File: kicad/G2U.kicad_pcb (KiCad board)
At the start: 2 copper layers, 78 x 71.4 mm, 38 parts, among them J1 Conn_02x12_Counter_Clockwise_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

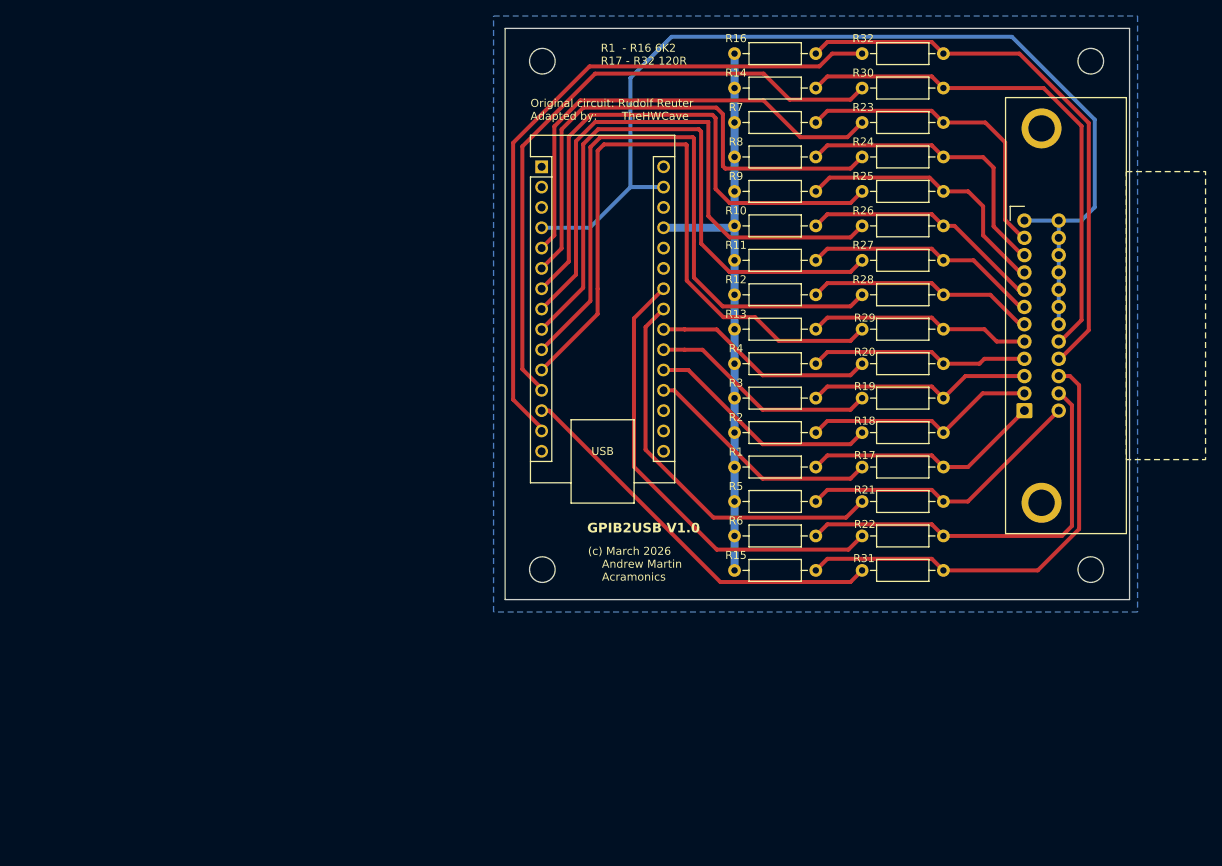
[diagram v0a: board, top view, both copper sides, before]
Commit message: Final 0603 board
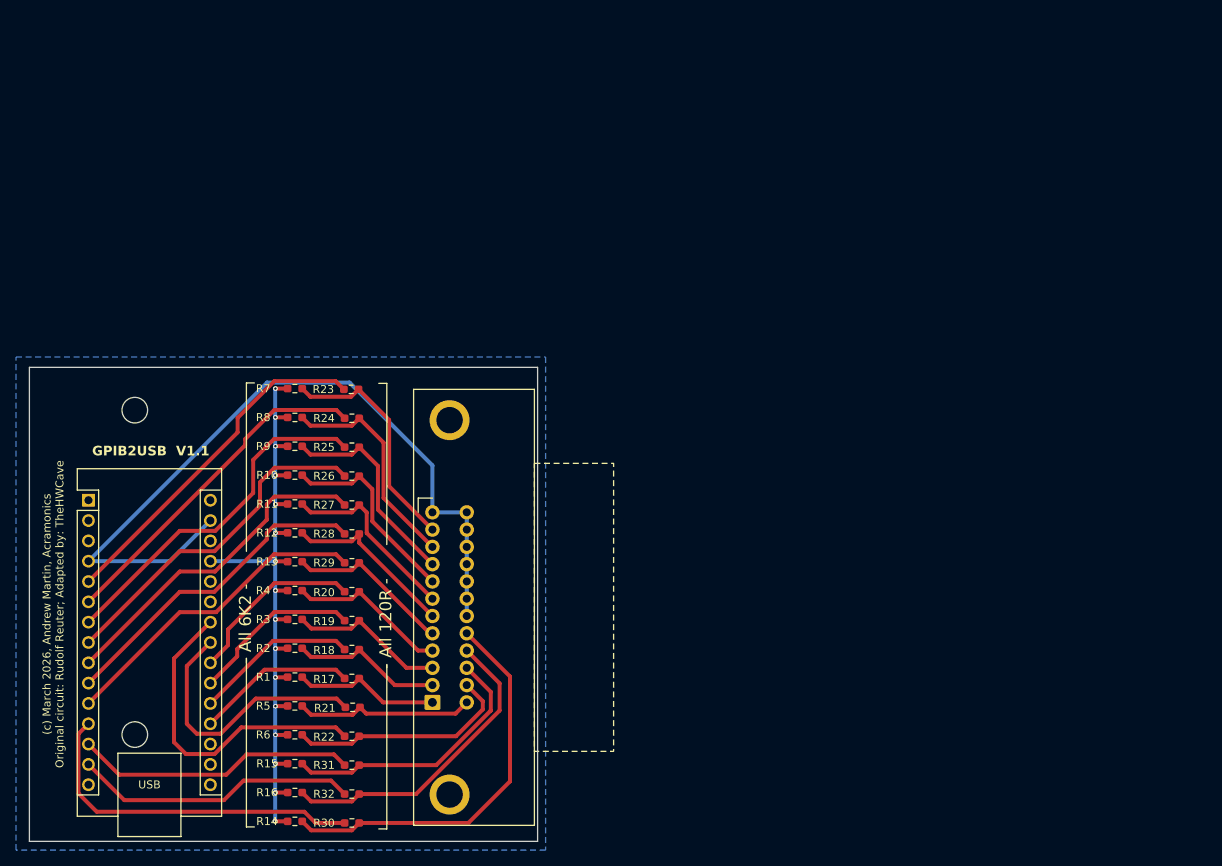
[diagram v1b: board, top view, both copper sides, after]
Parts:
- removed the REF** at (197.2, 34.1)
- removed the REF** at (197.2, 97.7)
- R1, R10, R11, R12, R13, R14, R15, R16, R17, R18, R19, R2, R20, R21, R22, R23, R24, R25, R26, R27, R28, R29, R3, R30, R31, R32, R4, R5, R6, R7, R8, R9: footprint Resistor_THT:R_Axial_DIN0207_L6.3mm_D2.5mm_P10.16mm_Horizontal -> Resistor_SMD:R_0603_1608Metric_Pad0.98x0.95mm_HandSolder
- moved R32 118.5 mm to (104.8, 125.8)
- moved R30 117.9 mm to (104.8, 129.4)
- moved R16 107.5 mm to (97.7, 125.6)
- moved R14 106.9 mm to (97.7, 129.2)
- moved J1 82.5 mm to (114.9, 90.5)
- moved R23 81.2 mm to (104.7, 75.2)
- moved R24 80.8 mm to (104.8, 78.8)
- moved R25 80.6 mm to (104.8, 82.4)
- moved R26 80.3 mm to (104.8, 86.0)
- moved R27 80.0 mm to (104.8, 89.6)
- moved R28 79.8 mm to (104.8, 93.2)
- moved R29 79.5 mm to (104.8, 96.8)
- moved R31 77.8 mm to (104.8, 122.1)
- moved A1 70.3 mm to (71.9, 89.0)
- moved R20 69.9 mm to (104.8, 100.5)
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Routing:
- net Net-(A1-D11): track 85.9 -> 35.6 mm
- net Net-(A1-D8): track 84.4 -> 40.2 mm
- net Net-(A1-D7): track 81.9 -> 41.1 mm
- net Net-(A1-D9): track 79.8 -> 44.0 mm
- net Net-(A1-D6): track 77.1 -> 42.2 mm
- net GND: track 128.8 -> 97.0 mm
- net Net-(J1-Pin_16): track 70.0 -> 39.0 mm
- net Net-(A1-D5): track 73.0 -> 43.2 mm
- net Net-(A1-D4): track 68.6 -> 44.4 mm
- net Net-(J1-Pin_15): track 57.3 -> 33.8 mm
- net Net-(J1-Pin_14): track 51.1 -> 28.7 mm
- net Net-(A1-D3): track 64.7 -> 42.8 mm
- net Net-(A1-A5): track 57.3 -> 40.7 mm
- net Net-(A1-A4): track 49.9 -> 34.0 mm
- net Net-(J1-Pin_17): track 64.6 -> 49.7 mm
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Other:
- board size 78 x 71.4 mm -> 63.5 x 59.2 mm
- board text added: "(c) March 2026, Andrew Martin, Acramonics Original circuit: Rudolf Reuter; Adapted by: TheHWCave"
- board text added: "- All 120R -"
- board text added: "- All 6K2 -"
- board text added: "GPIB2USB V1.1"
- board text removed: "(c) March 2026 Andrew Martin Acramonics"
- board text removed: "GPIB2USB V1.0"
- board text removed: "Original circuit: Rudolf Reuter Adapted by: TheHWCave"
- board text removed: "R1 - R16 6K2 R17 - R32 120R"
